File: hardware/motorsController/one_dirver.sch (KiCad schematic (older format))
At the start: 9 parts, among them U1 VNH5019A-E

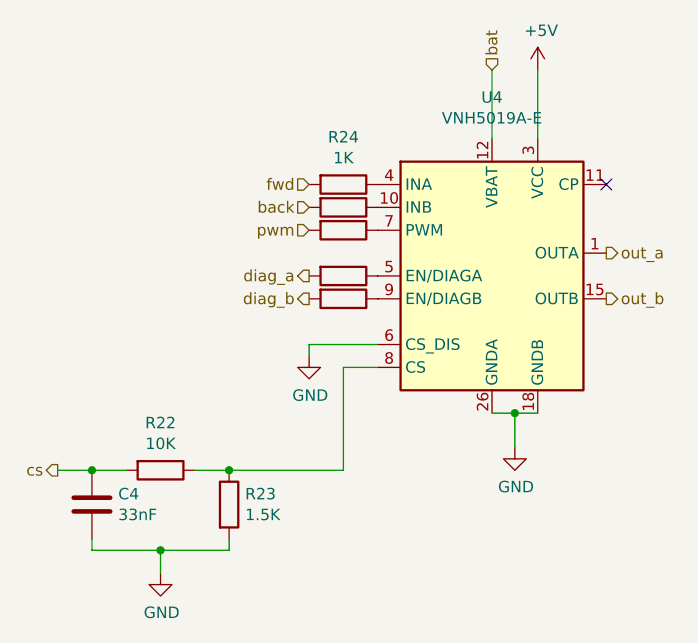
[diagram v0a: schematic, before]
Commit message: add a pull-up to encoder's output
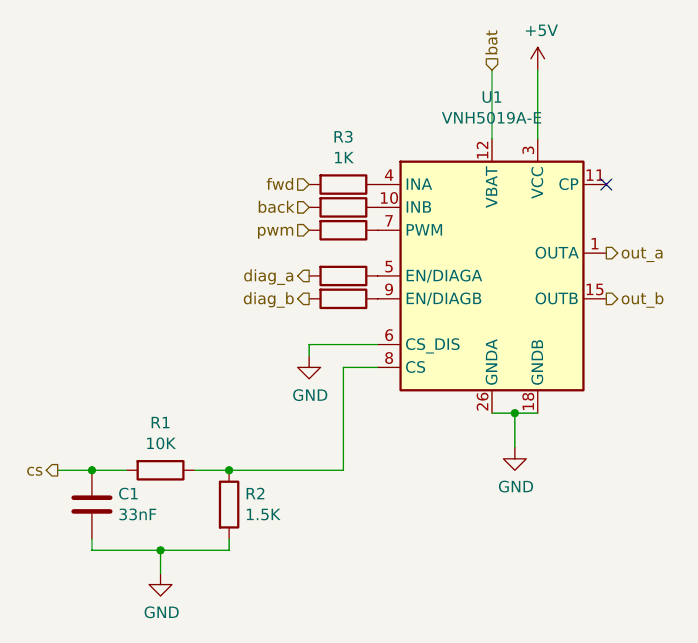
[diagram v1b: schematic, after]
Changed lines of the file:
@@
 AR Path="/5F8B7961/5F75DD74" Ref="U3"  Part="1"
 AR Path="/5F8B7981/5F75DD74" Ref="U4"  Part="1"
-F 0 "U4" H 3150 3531 50  0000 C CNN
+F 0 "U1" H 3150 3531 50  0000 C CNN
 F 1 "VNH5019A-E" H 3150 3440 50  0000 C CNN
 F 2 "Package_SO:ST_MultiPowerSO-30" H 4050 2200 50  0001 C CNN
@@
 AR Path="/5F8B7961/5F764A13" Ref="R17"  Part="1"
 AR Path="/5F8B7981/5F764A13" Ref="R24"  Part="1"
-F 0 "R24" V 2293 2350 50  0000 C CNN
+F 0 "R3" V 2293 2350 50  0000 C CNN
 F 1 "1K" V 2384 2350 50  0000 C CNN
 F 2 "Resistor_SMD:R_0805_2012Metric" V 2430 2350 50  0001 C CNN
@@
 AR Path="/5F8B7961/5F765406" Ref="R18"  Part="1"
 AR Path="/5F8B7981/5F765406" Ref="R25"  Part="1"
-F 0 "R25" V 2293 2450 50  0001 C CNN
+F 0 "R4" V 2293 2450 50  0001 C CNN
 F 1 "1K" V 2384 2450 50  0001 C CNN
 F 2 "Resistor_SMD:R_0805_2012Metric" V 2430 2450 50  0001 C CNN
@@
 AR Path="/5F8B7961/5F7658F2" Ref="R19"  Part="1"
 AR Path="/5F8B7981/5F7658F2" Ref="R26"  Part="1"
-F 0 "R26" V 2293 2550 50  0001 C CNN
+F 0 "R5" V 2293 2550 50  0001 C CNN
 F 1 "1K" V 2384 2550 50  0001 C CNN
 F 2 "Resistor_SMD:R_0805_2012Metric" V 2430 2550 50  0001 C CNN
@@
 AR Path="/5F8B7961/5F77E0ED" Ref="R20"  Part="1"
 AR Path="/5F8B7981/5F77E0ED" Ref="R27"  Part="1"
-F 0 "R27" V 2293 2750 50  0001 C CNN
+F 0 "R6" V 2293 2750 50  0001 C CNN
 F 1 "1K" V 2384 2750 50  0001 C CNN
 F 2 "Resistor_SMD:R_0805_2012Metric" V 2430 2750 50  0001 C CNN
@@
 AR Path="/5F8B7961/5F781639" Ref="R21"  Part="1"
 AR Path="/5F8B7981/5F781639" Ref="R28"  Part="1"
-F 0 "R28" V 2293 2850 50  0001 C CNN
+F 0 "R7" V 2293 2850 50  0001 C CNN
 F 1 "1K" V 2384 2850 50  0001 C CNN
 F 2 "Resistor_SMD:R_0805_2012Metric" V 2430 2850 50  0001 C CNN
@@
 AR Path="/5F8B7961/5F781B76" Ref="#PWR0112"  Part="1"
 AR Path="/5F8B7981/5F781B76" Ref="#PWR0116"  Part="1"
-F 0 "#PWR0116" H 2350 2850 50  0001 C CNN
+F 0 "#PWR0101" H 2350 2850 50  0001 C CNN
 F 1 "GND" H 2355 2927 50  0000 C CNN
 F 2 "" H 2350 3100 50  0001 C CNN
@@
 AR Path="/5F8B7961/5F782890" Ref="R16"  Part="1"
 AR Path="/5F8B7981/5F782890" Ref="R23"  Part="1"
-F 0 "R23" H 2070 3796 50  0000 L CNN
+F 0 "R2" H 2070 3796 50  0000 L CNN
 F 1 "1.5K" H 2070 3705 50  0000 L CNN
 F 2 "Resistor_SMD:R_0805_2012Metric" V 1930 3750 50  0001 C CNN
@@
 AR Path="/5F8B7961/5F783B44" Ref="#PWR0113"  Part="1"
 AR Path="/5F8B7981/5F783B44" Ref="#PWR0117"  Part="1"
-F 0 "#PWR0117" H 1700 3800 50  0001 C CNN
+F 0 "#PWR0102" H 1700 3800 50  0001 C CNN
 F 1 "GND" H 1705 3877 50  0000 C CNN
 F 2 "" H 1700 4050 50  0001 C CNN
@@
 AR Path="/5F8B7961/5F7841BA" Ref="R15"  Part="1"
 AR Path="/5F8B7981/5F7841BA" Ref="R22"  Part="1"
-F 0 "R22" V 1493 3600 50  0000 C CNN
+F 0 "R1" V 1493 3600 50  0000 C CNN
 F 1 "10K" V 1584 3600 50  0000 C CNN
 F 2 "Resistor_SMD:R_0805_2012Metric" V 1630 3600 50  0001 C CNN
@@
 AR Path="/5F8B7961/5F784D90" Ref="C3"  Part="1"
 AR Path="/5F8B7981/5F784D90" Ref="C4"  Part="1"
-F 0 "C4" H 1515 3796 50  0000 L CNN
+F 0 "C1" H 1515 3796 50  0000 L CNN
 F 1 "33nF" H 1515 3705 50  0000 L CNN
 F 2 "Capacitor_SMD:C_1206_3216Metric" H 1438 3600 50  0001 C CNN
@@
 AR Path="/5F8B7961/5F78A1BC" Ref="#PWR0114"  Part="1"
 AR Path="/5F8B7981/5F78A1BC" Ref="#PWR0118"  Part="1"
-F 0 "#PWR0118" H 3350 1700 50  0001 C CNN
+F 0 "#PWR0103" H 3350 1700 50  0001 C CNN
 F 1 "+5V" H 3365 2023 50  0000 C CNN
 F 2 "" H 3350 1850 50  0001 C CNN
@@
 AR Path="/5F8B7961/5F794080" Ref="#PWR0115"  Part="1"
 AR Path="/5F8B7981/5F794080" Ref="#PWR0119"  Part="1"
-F 0 "#PWR0119" H 3250 3250 50  0001 C CNN
+F 0 "#PWR0104" H 3250 3250 50  0001 C CNN
 F 1 "GND" H 3255 3327 50  0000 C CNN
 F 2 "" H 3250 3500 50  0001 C CNN

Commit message: remove RC filter from collector and add resisor  before emiter
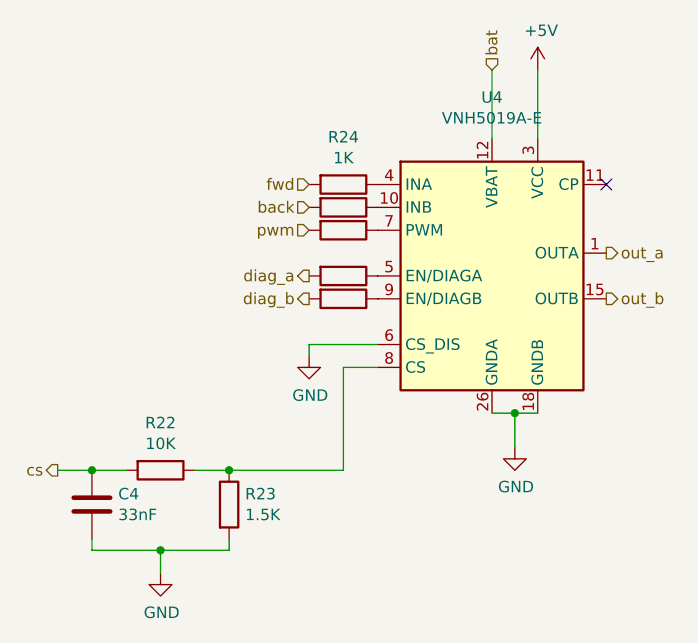
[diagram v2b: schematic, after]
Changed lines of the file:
@@
 AR Path="/5F8B7961/5F75DD74" Ref="U3"  Part="1"
 AR Path="/5F8B7981/5F75DD74" Ref="U4"  Part="1"
-F 0 "U1" H 3150 3531 50  0000 C CNN
+F 0 "U4" H 3150 3531 50  0000 C CNN
 F 1 "VNH5019A-E" H 3150 3440 50  0000 C CNN
 F 2 "Package_SO:ST_MultiPowerSO-30" H 4050 2200 50  0001 C CNN
@@
 AR Path="/5F8B7961/5F764A13" Ref="R17"  Part="1"
 AR Path="/5F8B7981/5F764A13" Ref="R24"  Part="1"
-F 0 "R3" V 2293 2350 50  0000 C CNN
+F 0 "R24" V 2293 2350 50  0000 C CNN
 F 1 "1K" V 2384 2350 50  0000 C CNN
 F 2 "Resistor_SMD:R_0805_2012Metric" V 2430 2350 50  0001 C CNN
@@
 AR Path="/5F8B7961/5F765406" Ref="R18"  Part="1"
 AR Path="/5F8B7981/5F765406" Ref="R25"  Part="1"
-F 0 "R4" V 2293 2450 50  0001 C CNN
+F 0 "R25" V 2293 2450 50  0001 C CNN
 F 1 "1K" V 2384 2450 50  0001 C CNN
 F 2 "Resistor_SMD:R_0805_2012Metric" V 2430 2450 50  0001 C CNN
@@
 AR Path="/5F8B7961/5F7658F2" Ref="R19"  Part="1"
 AR Path="/5F8B7981/5F7658F2" Ref="R26"  Part="1"
-F 0 "R5" V 2293 2550 50  0001 C CNN
+F 0 "R26" V 2293 2550 50  0001 C CNN
 F 1 "1K" V 2384 2550 50  0001 C CNN
 F 2 "Resistor_SMD:R_0805_2012Metric" V 2430 2550 50  0001 C CNN
@@
 AR Path="/5F8B7961/5F77E0ED" Ref="R20"  Part="1"
 AR Path="/5F8B7981/5F77E0ED" Ref="R27"  Part="1"
-F 0 "R6" V 2293 2750 50  0001 C CNN
+F 0 "R27" V 2293 2750 50  0001 C CNN
 F 1 "1K" V 2384 2750 50  0001 C CNN
 F 2 "Resistor_SMD:R_0805_2012Metric" V 2430 2750 50  0001 C CNN
@@
 AR Path="/5F8B7961/5F781639" Ref="R21"  Part="1"
 AR Path="/5F8B7981/5F781639" Ref="R28"  Part="1"
-F 0 "R7" V 2293 2850 50  0001 C CNN
+F 0 "R28" V 2293 2850 50  0001 C CNN
 F 1 "1K" V 2384 2850 50  0001 C CNN
 F 2 "Resistor_SMD:R_0805_2012Metric" V 2430 2850 50  0001 C CNN
@@
 AR Path="/5F8B7961/5F781B76" Ref="#PWR0112"  Part="1"
 AR Path="/5F8B7981/5F781B76" Ref="#PWR0116"  Part="1"
-F 0 "#PWR0101" H 2350 2850 50  0001 C CNN
+F 0 "#PWR0116" H 2350 2850 50  0001 C CNN
 F 1 "GND" H 2355 2927 50  0000 C CNN
 F 2 "" H 2350 3100 50  0001 C CNN
@@
 AR Path="/5F8B7961/5F782890" Ref="R16"  Part="1"
 AR Path="/5F8B7981/5F782890" Ref="R23"  Part="1"
-F 0 "R2" H 2070 3796 50  0000 L CNN
+F 0 "R23" H 2070 3796 50  0000 L CNN
 F 1 "1.5K" H 2070 3705 50  0000 L CNN
 F 2 "Resistor_SMD:R_0805_2012Metric" V 1930 3750 50  0001 C CNN
@@
 AR Path="/5F8B7961/5F783B44" Ref="#PWR0113"  Part="1"
 AR Path="/5F8B7981/5F783B44" Ref="#PWR0117"  Part="1"
-F 0 "#PWR0102" H 1700 3800 50  0001 C CNN
+F 0 "#PWR0117" H 1700 3800 50  0001 C CNN
 F 1 "GND" H 1705 3877 50  0000 C CNN
 F 2 "" H 1700 4050 50  0001 C CNN
@@
 AR Path="/5F8B7961/5F7841BA" Ref="R15"  Part="1"
 AR Path="/5F8B7981/5F7841BA" Ref="R22"  Part="1"
-F 0 "R1" V 1493 3600 50  0000 C CNN
+F 0 "R22" V 1493 3600 50  0000 C CNN
 F 1 "10K" V 1584 3600 50  0000 C CNN
 F 2 "Resistor_SMD:R_0805_2012Metric" V 1630 3600 50  0001 C CNN
@@
 AR Path="/5F8B7961/5F784D90" Ref="C3"  Part="1"
 AR Path="/5F8B7981/5F784D90" Ref="C4"  Part="1"
-F 0 "C1" H 1515 3796 50  0000 L CNN
+F 0 "C4" H 1515 3796 50  0000 L CNN
 F 1 "33nF" H 1515 3705 50  0000 L CNN
 F 2 "Capacitor_SMD:C_1206_3216Metric" H 1438 3600 50  0001 C CNN
@@
 AR Path="/5F8B7961/5F78A1BC" Ref="#PWR0114"  Part="1"
 AR Path="/5F8B7981/5F78A1BC" Ref="#PWR0118"  Part="1"
-F 0 "#PWR0103" H 3350 1700 50  0001 C CNN
+F 0 "#PWR0118" H 3350 1700 50  0001 C CNN
 F 1 "+5V" H 3365 2023 50  0000 C CNN
 F 2 "" H 3350 1850 50  0001 C CNN
@@
 AR Path="/5F8B7961/5F794080" Ref="#PWR0115"  Part="1"
 AR Path="/5F8B7981/5F794080" Ref="#PWR0119"  Part="1"
-F 0 "#PWR0104" H 3250 3250 50  0001 C CNN
+F 0 "#PWR0119" H 3250 3250 50  0001 C CNN
 F 1 "GND" H 3255 3327 50  0000 C CNN
 F 2 "" H 3250 3500 50  0001 C CNN
